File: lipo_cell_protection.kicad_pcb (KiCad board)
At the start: 2 copper layers, 9.3 x 5.8 mm, 12 parts, among them J1 V_CELL, J2 GND_CELL, J3 V_CELL, J4 V_CELL, Q1 PMZ600UNEYL, Q2 PMZ600UNEYL, U1 BQ29700DSER

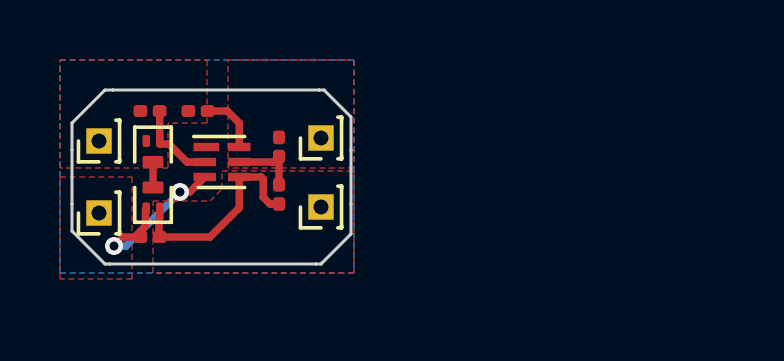
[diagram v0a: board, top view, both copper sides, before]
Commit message: round attempt
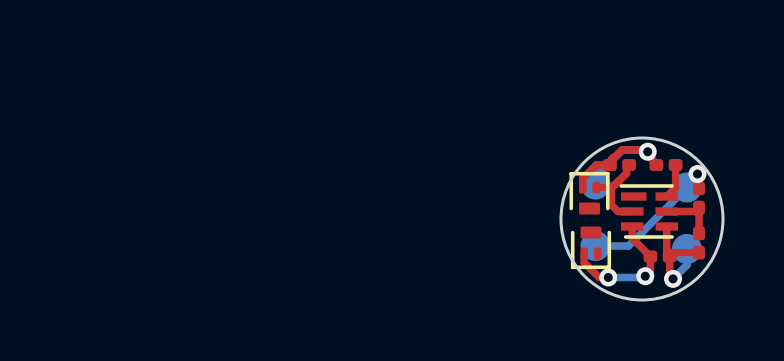
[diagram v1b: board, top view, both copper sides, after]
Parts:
- J1, J2, J3, J4: footprint Connector_PinHeader_1.00mm:PinHeader_1x01_P1.00mm_Vertical -> TestPoint:TestPoint_Pad_D1.0mm; moved to B.Cu
- moved R2 17.0 mm to (39.2, 29.6)
- moved J4 16.6 mm to (37.0, 27.2)
- moved J3 16.6 mm to (37.0, 29.3)
- moved R3 15.8 mm to (37.9, 26.6)
- moved R4 15.7 mm to (39.4, 26.6)
- moved Q1 14.7 mm to (36.9, 29.2)
- moved Q2 14.6 mm to (36.9, 27.7)
- moved U1 14.3 mm to (38.9, 28.1)
- moved R1 14.1 mm to (40.5, 27.7)
- moved C1 14.1 mm to (40.5, 29.2)
- moved J1 12.3 mm to (40.1, 27.4)
- moved J2 12.3 mm to (40.1, 29.4)
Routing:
- net GND: track 0.00 -> 6.44 mm, vias 0 -> 1
- net +BATT: track 0.00 -> 4.45 mm, vias 0 -> 1
- net -BATT: track 6.96 -> 3.87 mm, vias 0 -> 1
- net Net-(Q1-G): track 6.01 -> 4.54 mm
- net Net-(Q1-D): track 0.75 -> 0.00 mm
- net Net-(U1-V-): track 1.92 -> 1.17 mm
- removed copper zone on B.Cu, net +BATT
- removed copper zone on F.Cu, net +BATT
- removed copper zone on F.Cu, net -BATT
- removed copper zone on F.Cu, net GND
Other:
- board size 9.3 x 5.8 mm -> 5.4 x 5.4 mm

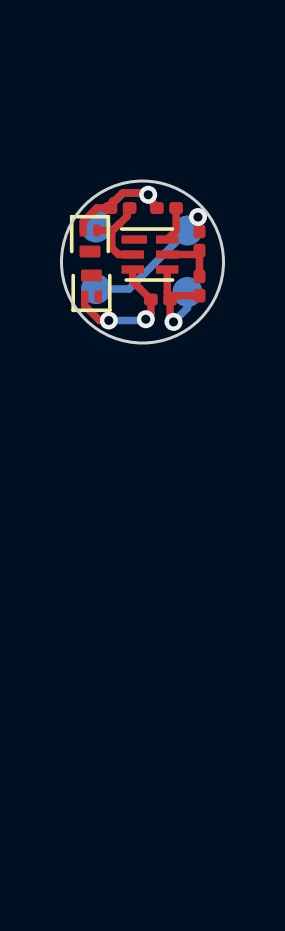
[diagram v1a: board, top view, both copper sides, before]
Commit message: full
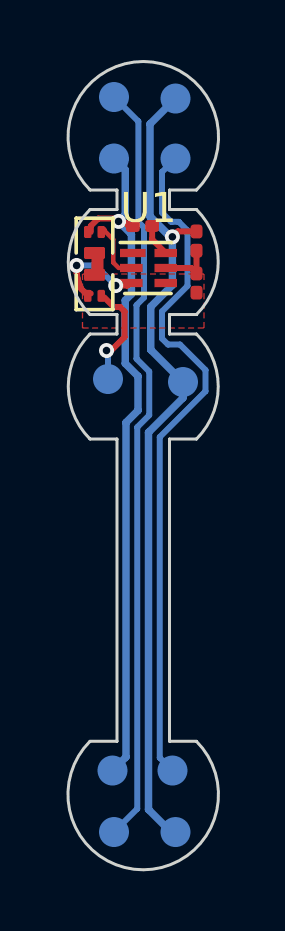
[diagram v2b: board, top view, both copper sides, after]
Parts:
- removed R2, R3: 5M, Resistor_SMD:R_0201_0603Metric
- added J10: SIG_2, TestPoint:TestPoint_Pad_D1.0mm, B.Cu at (39.7, 24.9)
- added J5: VCC, TestPoint:TestPoint_Pad_D1.0mm, B.Cu at (39.7, 47.4)
- added J6: GND, TestPoint:TestPoint_Pad_D1.0mm, B.Cu at (37.6, 45.4)
- added J7: SIG_1, TestPoint:TestPoint_Pad_D1.0mm, B.Cu at (37.6, 47.4)
- added J8: SIG_2, TestPoint:TestPoint_Pad_D1.0mm, B.Cu at (39.6, 45.4)
- added J9: SIG_1, TestPoint:TestPoint_Pad_D1.0mm, B.Cu at (37.6, 22.9)
- J3: value V_CELL -> VCC
- J4: value V_CELL -> GND
- moved J3 6.88 mm to (39.7, 22.9), turned to 180 degrees
- moved J1 5.05 mm to (40.0, 32.4)
- moved J2 3.93 mm to (37.5, 32.3)
- moved J4 2.38 mm to (37.6, 24.9), turned to 180 degrees
- moved R4 1.00 mm to (38.6, 27.2)
- moved U1 0.45 mm to (38.8, 28.6)
- moved Q2 0.16 mm to (37.0, 27.8)
- moved C1 0.14 mm to (40.4, 29.1)
- moved Q1 0.10 mm to (37.0, 29.2)
- moved R1 0.10 mm to (40.4, 27.7)
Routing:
- net /SIG_1: track 0.00 -> 25.7 mm
- net +BATT: track 4.45 -> 29.0 mm
- net /SIG_2: track 0.00 -> 23.1 mm
- net GND: track 6.44 -> 24.0 mm
- net Net-(Q1-G): track 4.54 -> 3.27 mm
- net Net-(Q2-G): track 3.10 -> 2.00 mm
- net Net-(Q1-D): track 0.00 -> 0.65 mm
- added copper zone on F.Cu, net -BATT
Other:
- board size 5.4 x 5.4 mm -> 5 x 26.9 mm
- board text added: "Connector goes on the bottom"
- board text added: "SMD"
- board text added: "Solder battery cables or electrodes on the bottom"
- board text added: "TH"
- board text added: "Total height: - Flex PCB thickness : 0.1 * 3 = 0.3 - Components : 0.8 - stiffener: 0.1 * 3 = 0.3 (stiffener or battery cables connections optional) - electrode or cable solder: 0.3 Total: 1.5 - 1.7mm + connector height"
